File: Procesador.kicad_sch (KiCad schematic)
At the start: 62 parts, among them CN1 10way 1.27mm, J8 Micro_SD_Card_Det1, J9 RJ45_Wuerth_7499010211A, SW1 Reset, U20 24AA02E-OT, U21 FT900Q, U22 MCP9700Ax-ETT, Y1 Crystal, Y2 Crystal

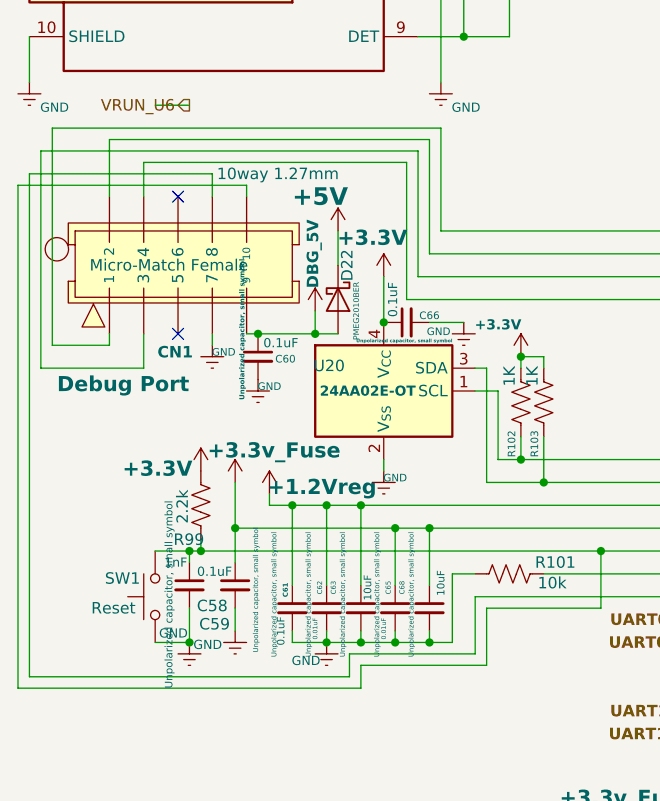
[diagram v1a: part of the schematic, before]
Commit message: 21-JUL-26
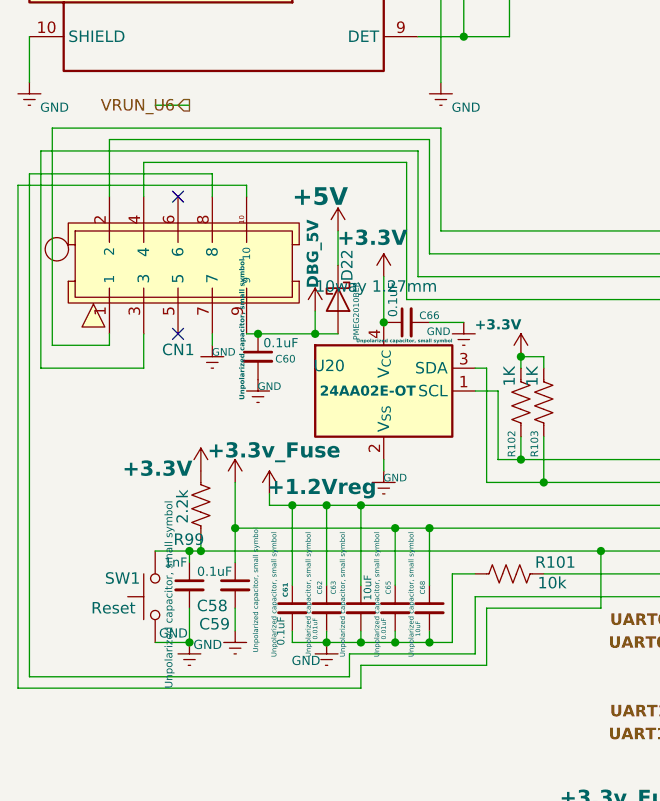
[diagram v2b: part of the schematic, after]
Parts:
- C68: footprint (none) -> Capacitor_SMD:C_0603_1608Metric_Pad1.08x0.95mm_HandSolder
- CN1: Field8 Micro-Match Female -> (none); Field9 Debug Port -> (none)
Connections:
- net DBG_5V: now also CN1.9; no longer CN1. (9)
- net GND: now also CN1.7; no longer CN1. (9)
- net at C58.1, R99.1, SW1.2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: now also CN1.10; no longer CN1. (9)
- net at U21.20 (SPIS0_CLK/GPIO36): now also CN1.1; no longer CN1. (9)
- net at U21.21 (SPIS0_SS/GPIO37): now also CN1.2; no longer CN1. (9)
- net at U21.22 (SPIS0_MOSI/GPIO38): now also CN1.3; no longer CN1. (9)
- net at U21.23 (SPIS0_MISO/GPIO39): now also CN1.4; no longer CN1. (9)
- net at U21.36 (DEBUG): now also CN1.8; no longer CN1. (9)
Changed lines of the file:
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@@
 	)
 	(symbol
-		(lib_id "CONECTORES GRACIDA:1-215079-0_microMatch10P_1.27mm")
-		(at 19.05 71.12 0)
-		(unit 1)
-		(exclude_from_sim no)
-		(in_bom yes)
-		(on_board yes)
-		(dnp no)
-		(property "Reference" "CN1"
-			(at 28.194 84.582 0)
-			(effects
-				(font
-					(size 1.27 1.27)
-					(thickness 0.254)
-					(bold yes)
-				)
-				(justify left)
-			)
-		)
-		(property "Value" "10way 1.27mm"
-			(at 34.798 64.77 0)
-			(effects
-				(font
-					(size 1.27 1.27)
-				)
-				(justify left)
-			)
-		)
-		(property "Footprint" "CONECTORES GRACIDA:MicroMatch_10way_P1.75mm"
-			(at 38.608 59.69 0)
-			(effects
-				(font
-					(size 1.27 1.27)
-				)
-				(hide yes)
-			)
-		)
-		(property "Datasheet" "https://www.te.com/commerce/DocumentDelivery/DDEController?Action=srchrtrv&DocNm=215079&DocType=Customer+Drawing&DocLang=English&PartCntxt=1-215079-0&DocFormat=pdf"
-			(at 24.13 55.88 0)
-			(effects
-				(font
-					(size 1.27 1.27)
-				)
-				(hide yes)
-			)
-		)
-		(property "Description" "10way 1.27mm microMatch"
-			(at 28.448 87.63 0)
-			(effects
-				(font
-					(size 1.27 1.27)
-				)
-				(hide yes)
-			)
-		)
-		(property "Mouser" "571-12150790"
-			(at 18.542 61.976 0)
-			(effects
-				(font
-					(size 1.27 1.27)
-				)
-				(hide yes)
-			)
-		)
-		(property "Digikey" "17-1-215079-0TR-ND"
-			(at 26.416 90.17 0)
-			(effects
-				(font
-					(size 1.27 1.27)
-				)
-				(hide yes)
-			)
-		)
-		(property "Price" "1.14"
-			(at 14.986 64.008 0)
-			(effects
-				(font
-					(size 1.27 1.27)
-				)
-				(hide yes)
-			)
-		)
-		(property "Field8" "Micro-Match Female"
-			(at 29.464 74.93 0)
-			(effects
-				(font
-					(size 1.27 1.27)
-					(color 255 255 0 1)
-				)
-			)
-		)
-		(property "Field9" "Debug Port"
-			(at 24.384 88.138 0)
-			(effects
-				(font
-					(size 1.6764 1.6764)
-					(thickness 0.3353)
-					(bold yes)
-				)
-			)
-		)
-		(pin ""
-		)
-		(pin ""
-		)
-		(pin ""
-		)
-		(pin ""
-		)
-		(pin ""
-		)
-		(pin ""
-		)
-		(pin ""
-		)
-		(pin ""
-		)
-		(pin ""
-		)
-		(pin ""
-		)
-		(instances
-			(project ""
-				(path "/38a2da3c-ed29-422f-ab41-066ccf490e61/47b626b2-f3da-43c3-a614-3ce0196b783a"
-					(reference "CN1")
-					(unit 1)
-				)
-			)
-		)
-	)
-	(symbol
 		(lib_id "power:GNDREF")
 		(at 267.97 90.17 0)
@@
 	)
 	(symbol
-		(lib_id "Device:C_Small")
-		(at 58.42 113.03 0)
-		(unit 1)
-		(exclude_from_sim no)
-		(in_bom yes)
-		(on_board yes)
-		(dnp no)
-		(property "Reference" "C68"
-			(at 55.372 110.744 90)
-			(effects
-				(font
-					(size 0.5588 0.5588)
-				)
-			)
-		)
-		(property "Value" "10uF"
-			(at 59.69 110.236 90)
-			(effects
-				(font
-					(size 0.8382 0.8382)
-				)
-			)
-		)
-		(property "Footprint" ""
-			(at 58.42 113.03 0)
-			(effects
-				(font
-					(size 1.27 1.27)
-				)
-				(hide yes)
-			)
-		)
-		(property "Datasheet" "~"
-			(at 58.42 113.03 0)
-			(effects
-				(font
-					(size 1.27 1.27)
-				)
-				(hide yes)
-			)
-		)
-		(property "Description" "Unpolarized capacitor, small symbol"
-			(at 56.388 111.506 90)
-			(effects
-				(font
-					(size 0.5588 0.5588)
-				)
-			)
-		)
-		(pin "2"
-		)
-		(pin "1"
-		)
-		(instances
-			(project "01_IO-ASD-PLUS"
-				(path "/38a2da3c-ed29-422f-ab41-066ccf490e61/47b626b2-f3da-43c3-a614-3ce0196b783a"
-					(reference "C68")
-					(unit 1)
-				)
-			)
-		)
-	)
-	(symbol
 		(lib_id "Device:R_US")
 		(at 203.2 60.96 270)
@@
 	)
 	(symbol
+		(lib_name "1-215079-0_microMatch10P_1.27mm_1")
+		(lib_id "CONECTORES GRACIDA:1-215079-0_microMatch10P_1.27mm")
+		(at 19.05 71.12 0)
+		(unit 1)
+		(exclude_from_sim no)
+		(in_bom yes)
+		(on_board yes)
+		(dnp no)
+		(property "Reference" "CN1"
+			(at 28.702 84.328 0)
+			(effects
+				(font
+					(size 1.27 1.27)
+				)
+				(justify left)
+			)
+		)
+		(property "Value" "10way 1.27mm"
+			(at 45.72 77.2794 0)
+			(effects
+				(font
+					(size 1.27 1.27)
+				)
+				(justify left)
+			)
+		)
+		(property "Footprint" "CONECTORES GRACIDA:MicroMatch_10way_P1.75mm"
+			(at 38.608 59.69 0)
+			(effects
+				(font
+					(size 1.27 1.27)
+				)
+				(hide yes)
+			)
+		)
+		(property "Datasheet" "https://www.te.com/commerce/DocumentDelivery/DDEController?Action=srchrtrv&DocNm=215079&DocType=Customer+Drawing&DocLang=English&PartCntxt=1-215079-0&DocFormat=pdf"
+			(at 24.13 55.88 0)
+			(effects
+				(font
+					(size 1.27 1.27)
+				)
+				(hide yes)
+			)
+		)
+		(property "Description" "10way 1.27mm microMatch"
+			(at 28.448 87.63 0)
+			(effects
+				(font
+					(size 1.27 1.27)
+				)
+				(hide yes)
+			)
+		)
+		(property "Mouser" "571-12150790"
+			(at 18.542 61.976 0)
+			(effects
+				(font
+					(size 1.27 1.27)
+				)
+				(hide yes)
+			)
+		)
+		(property "Digikey" "17-1-215079-0TR-ND"
+			(at 26.416 90.17 0)
+			(effects
+				(font
+					(size 1.27 1.27)
+				)
+				(hide yes)
+			)
+		)
+		(property "Price" "1.14"
+			(at 14.986 64.008 0)
+			(effects
+				(font
+					(size 1.27 1.27)
+				)
+				(hide yes)
+			)
+		)
+		(pin "8"
+		)
+		(pin "9"
+		)
+		(pin "1"
+		)
+		(pin "4"
+		)
+		(pin "6"
+		)
+		(pin "5"
+		)
+		(pin "7"
+		)
+		(pin "2"
+		)
+		(pin "3"
+		)
+		(pin "10"
+		)
+		(instances
+			(project ""
+				(path "/38a2da3c-ed29-422f-ab41-066ccf490e61/47b626b2-f3da-43c3-a614-3ce0196b783a"
+					(reference "CN1")
+					(unit 1)
+				)
+			)
+		)
+	)
+	(symbol
 		(lib_id "power:+3.3V")
 		(at 273.05 73.66 0)
@@
 					(unit 1)
 				)
+			)
+		)
+	)
+	(symbol
+		(lib_id "Device:C_Small")
+		(at 58.42 113.03 0)
+		(unit 1)
+		(exclude_from_sim no)
+		(in_bom yes)
+		(on_board yes)
+		(dnp no)
+		(property "Reference" "C68"
+			(at 57.658 110.744 90)
+			(effects
+				(font
+					(size 0.5588 0.5588)
+				)
+			)
+		)
+		(property "Value" "10uF"
+			(at 57.15 115.316 90)
+			(effects
+				(font
+					(size 0.508 0.508)
+				)
+			)
+		)
+		(property "Footprint" "Capacitor_SMD:C_0603_1608Metric_Pad1.08x0.95mm_HandSolder"
+			(at 58.42 113.03 0)
+			(effects
+				(font
+					(size 1.27 1.27)
+				)
+				(hide yes)
+			)
+		)
+		(property "Datasheet" "~"
+			(at 58.42 113.03 0)
+			(effects
+				(font
+					(size 1.27 1.27)
+				)
+				(hide yes)
+			)
+		)
+		(property "Description" "Unpolarized capacitor, small symbol"
+			(at 56.388 111.506 90)
+			(effects
+				(font
+					(size 0.5588 0.5588)
+				)
+			)
+		)
+		(pin "2"
+		)
+		(pin "1"
+		)
+		(instances
+			(project "01_IO-ASD-PLUS"
+				(path "/38a2da3c-ed29-422f-ab41-066ccf490e61/47b626b2-f3da-43c3-a614-3ce0196b783a"
+					(reference "C68")
+					(unit 1)
+				)
